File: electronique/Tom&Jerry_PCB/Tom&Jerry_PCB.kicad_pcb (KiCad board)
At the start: 4 copper layers, 54 x 57 mm, 146 parts, among them IC1101 NCS199A2RSQT2G, IC301 TCA9555RTWR, IC901 NCS199A2RSQT2G, J1001 FTSH-105-01-F-DV-P-TR, J1301 Conn_01x02, J1501 Conn_01x02, J1601 Conn_01x02, J1701 Conn_01x02, J201 Interrupteur, J202 USB_C_Receptacle_USB2.0_16P, J203 Conn_01x02, J204 Conn_01x02, J301 Conn_01x08, J401 Conn_01x06, J402 Conn_01x06, J501 Conn_ST_STDC14, J601 Conn_01x03, J701 FTSH-105-01-F-DV-P-TR, Q201 SI2365EDS-T1-GE3, SW501 SW_Push, SW502 SW_Push, SW503 SW_Push, U1101 ZXBM5210-S, U201 MP1475DJ-LF-P, U202 BQ25172DSGR, U301 ADXL343, U501 STM32G431CBU6, U601 PAM8302AAY, U801 LP5812ADSDR, U901 ZXBM5210-S, Y501 16MHz

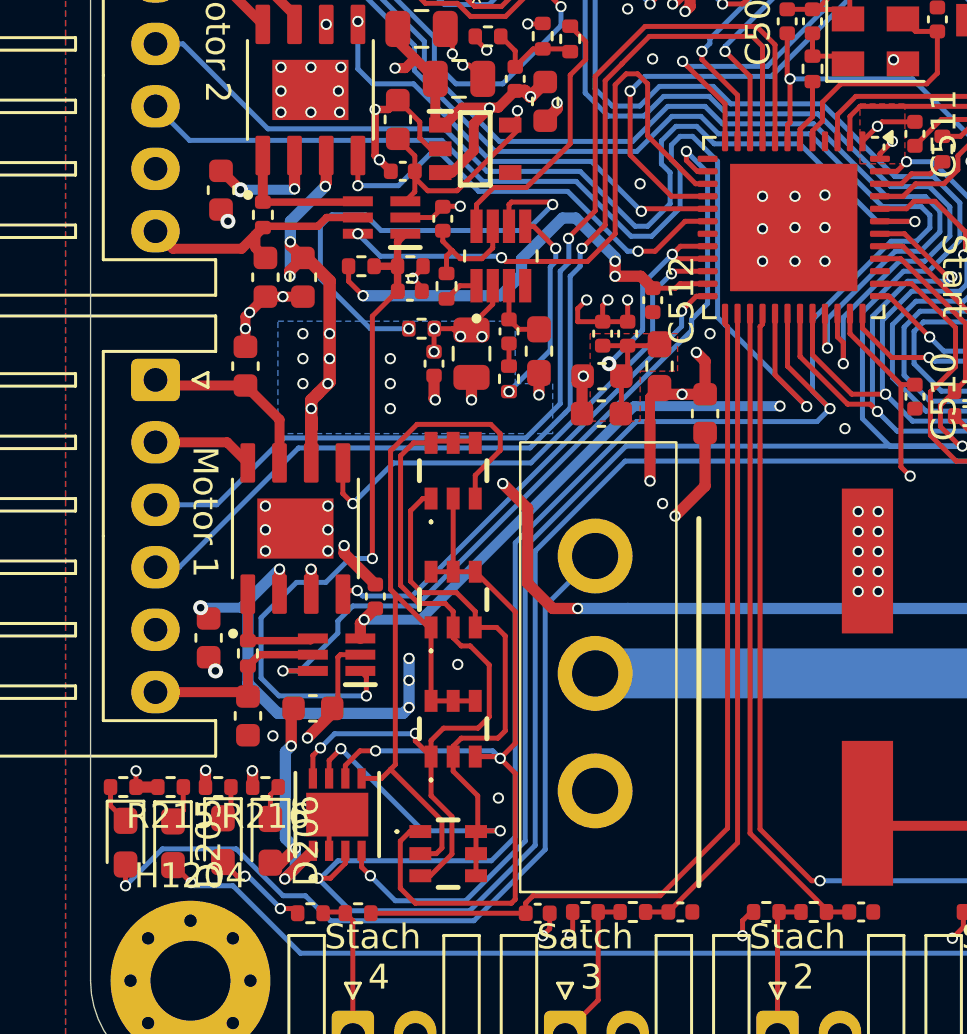
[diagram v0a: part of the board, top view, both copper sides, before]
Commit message: Derniere modif jlcpcb
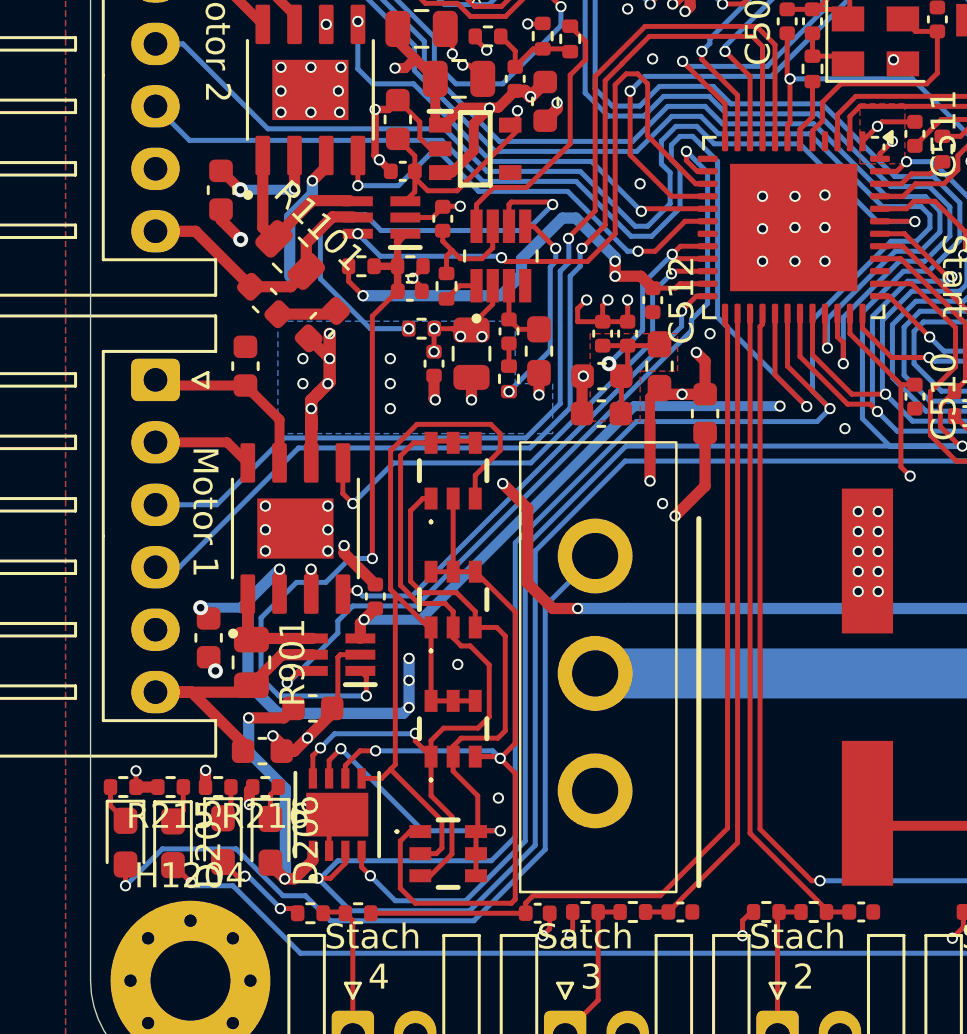
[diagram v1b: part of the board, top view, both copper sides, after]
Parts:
- R1101, R901: footprint Resistor_SMD:R_0402_1005Metric -> Resistor_SMD:R_0805_2012Metric
- moved C1102 2.05 mm to (83.3, 84.1), turned to 45 degrees
- moved R1101 1.94 mm to (82.0, 81.3), turned to -45 degrees
- moved C903 1.52 mm to (80.9, 101.2), turned to 0 degrees
- moved C1103 0.93 mm to (81.0, 83.2), turned to -45 degrees
- moved R901 0.39 mm to (80.4, 97.7)
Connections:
- U1101 pad 9: (no net) -> GND
- U202 pad 10: (no net) -> GND
- U202 pad 11: (no net) -> GND
- U601 pad 9: (no net) -> GND
- U901 pad 9: (no net) -> GND
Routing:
- net /Motors&Drivers/Motor1+: track 7.78 -> 11.8 mm
- net +5V: track 120.5 -> 117.8 mm, vias 34 -> 30
- net GND: track 122.4 -> 124.6 mm, vias 104 -> 101
- net Net-(IC1101-IN+): track 5.68 -> 7.19 mm
